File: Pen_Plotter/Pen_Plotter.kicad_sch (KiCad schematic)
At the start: 36 parts, among them J1 USB4125-GF-A_REVA2, J2 Motor 1, J3 Motor 2, J4 Servo, J5 6120XX21621_61200621621, J6 Y Lim, J8 X Lim, SW1 Reset-EN, SW2 Boot-GPIO0, U1 ESP32-WROOM-32E, U2 Regulator_Linear_3.3V_1A_Diod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, U4 ULN2803

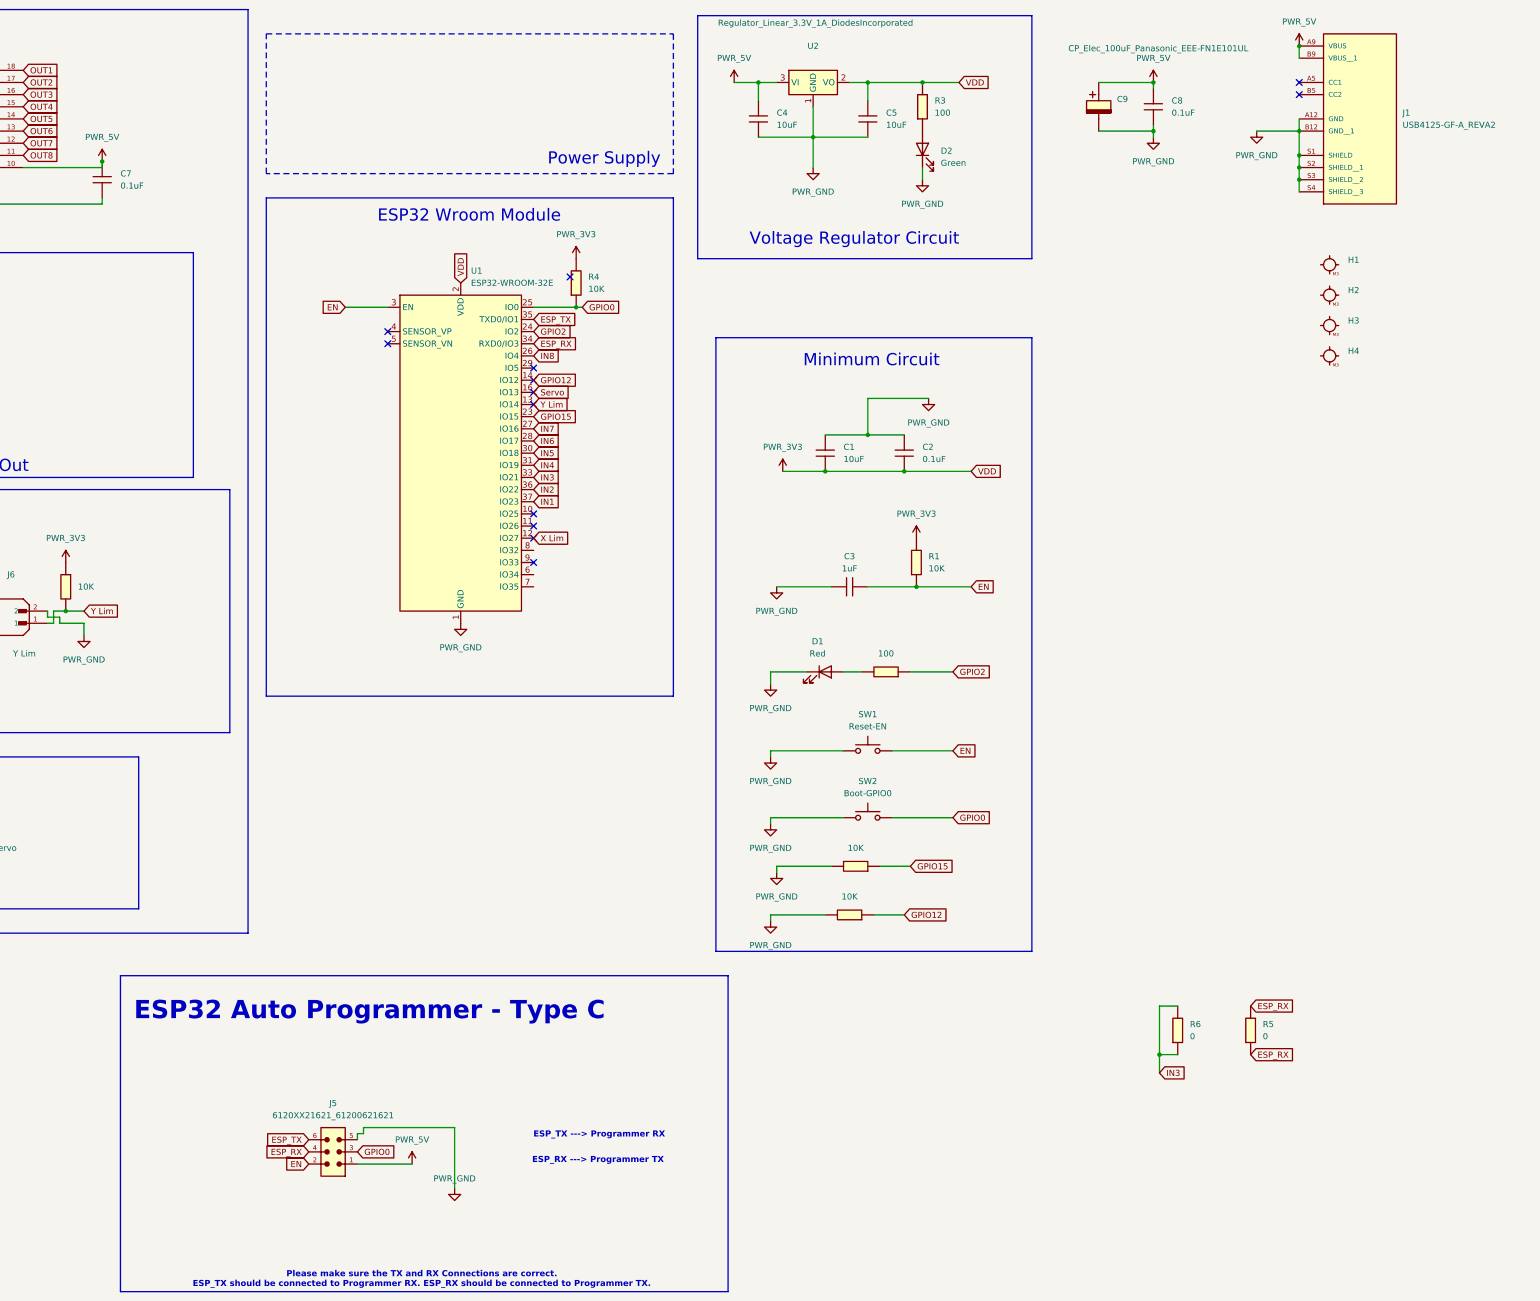
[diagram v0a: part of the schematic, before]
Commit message: updated readme file
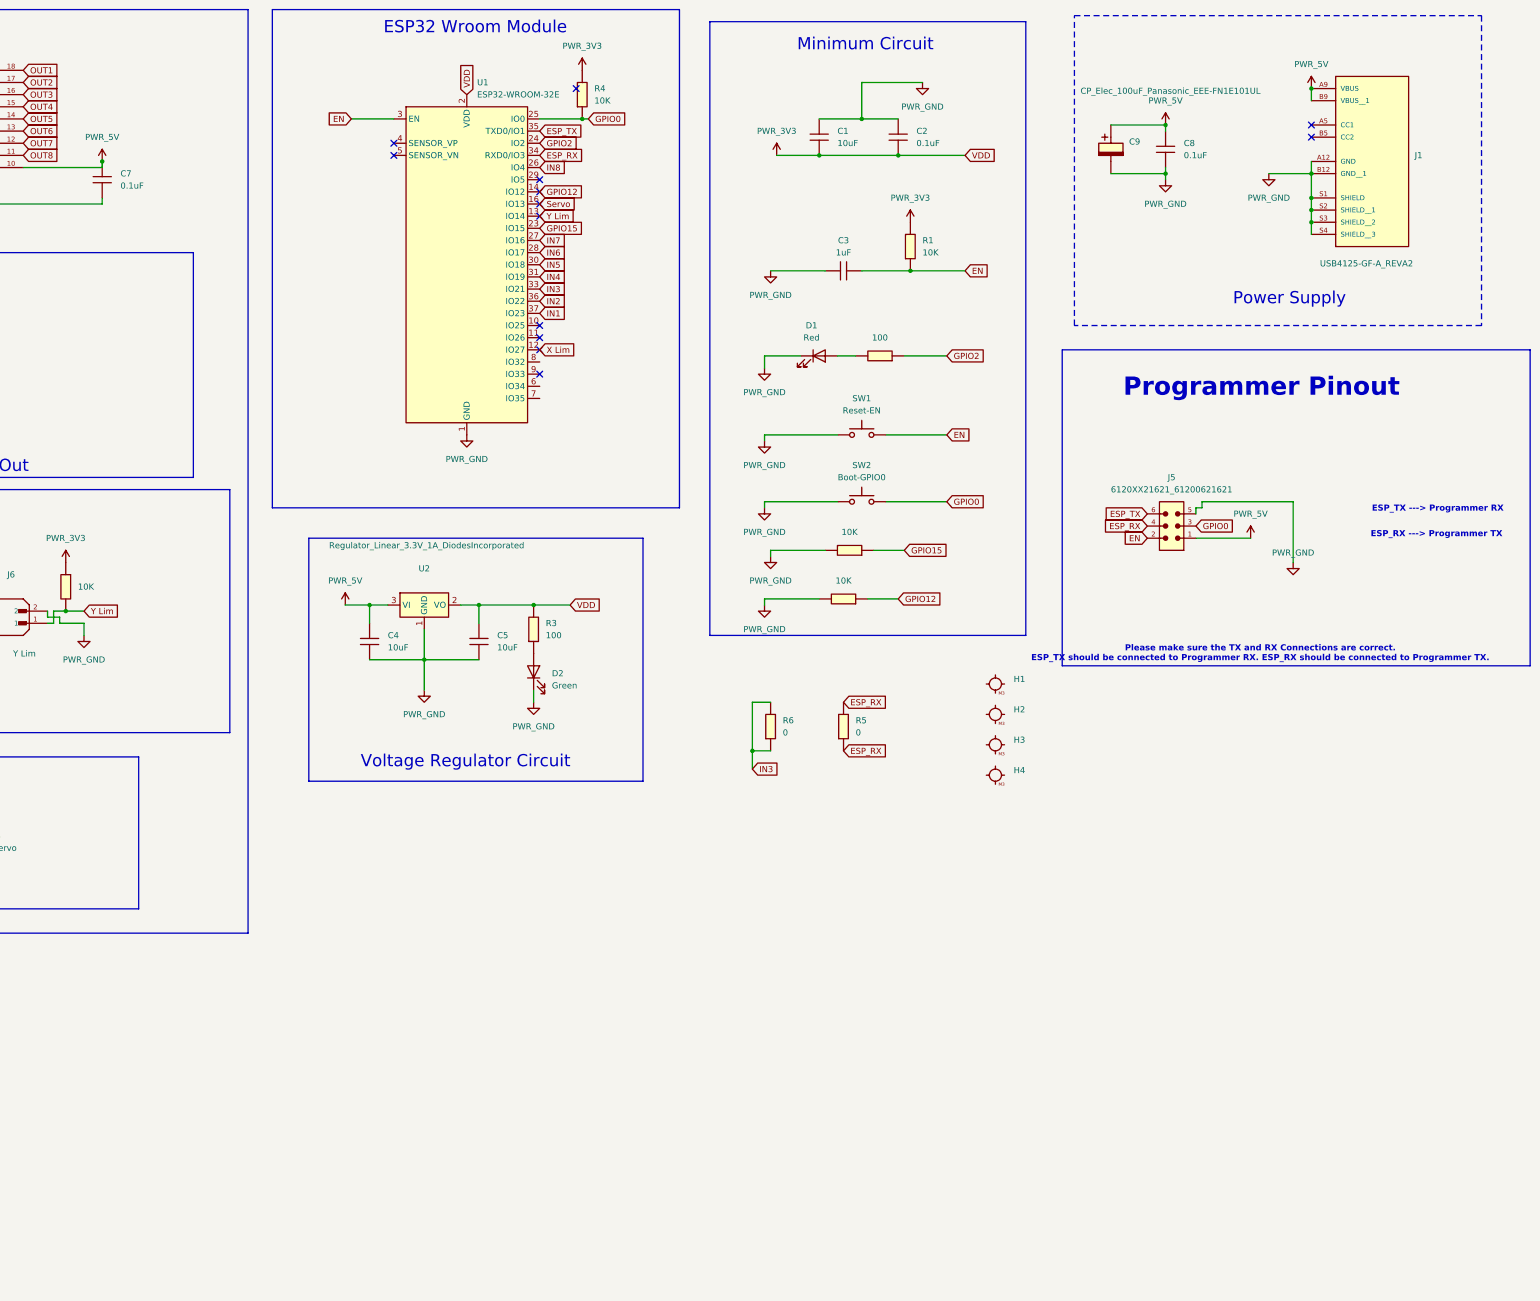
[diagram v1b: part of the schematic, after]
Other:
- note added: "Programmer Pinout"
- note removed: "ESP32 Auto Programmer - Type C"
- moved on the sheet: C1, C2, C3, C4, C5, C8, C9, D1, D2, H1, H2, H3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
